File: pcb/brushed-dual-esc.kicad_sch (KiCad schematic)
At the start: 2 parts, among them J3 Conn_ARM_JTAG_SWD_10, U3 STM32C011F4Ux

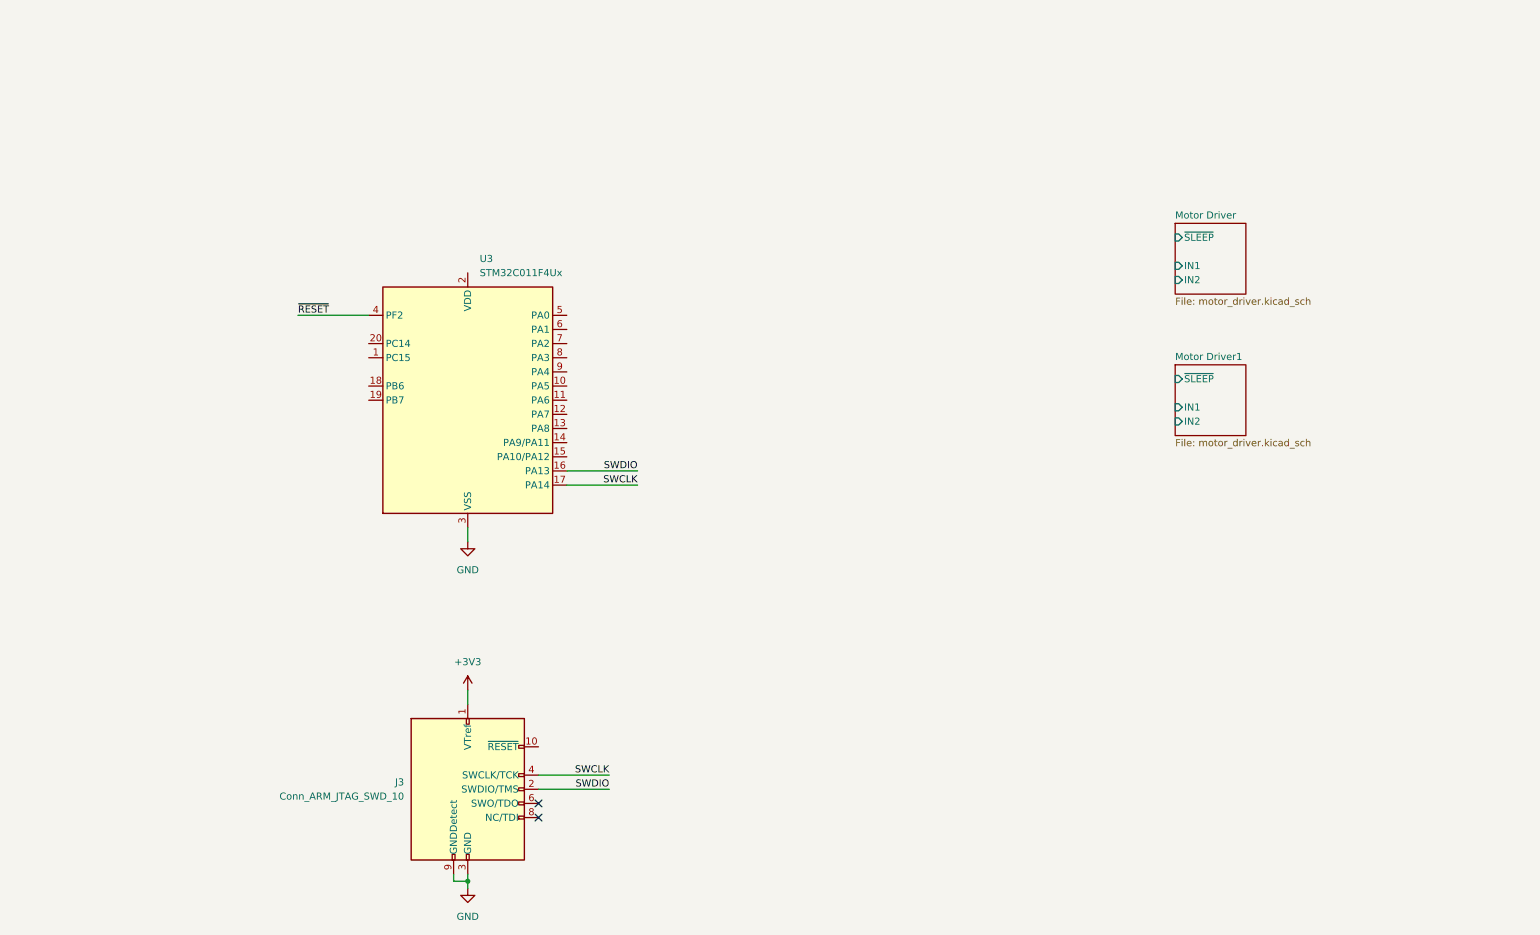
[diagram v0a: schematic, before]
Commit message: Finish design
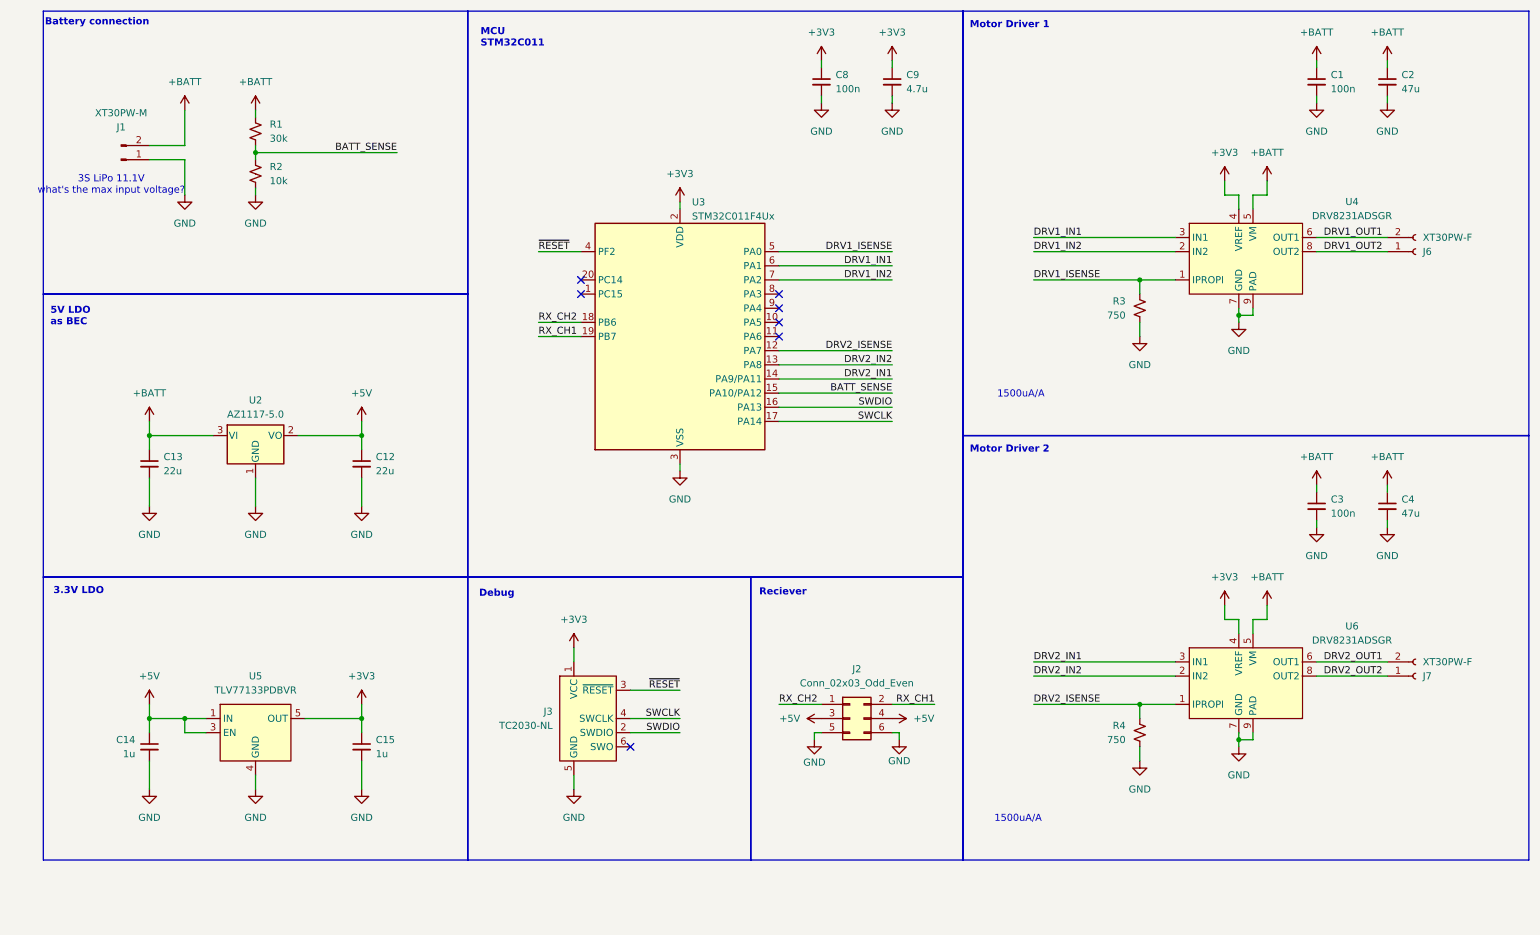
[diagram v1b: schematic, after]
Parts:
- removed J3: Conn_ARM_JTAG_SWD_10, Connector_PinHeader_1.27mm:PinHeader_2x05_P1.27mm_Vertical, symbol Connector:Conn_ARM_JTAG_SWD_10
- added C1, C3, C8: 100n, Capacitor_SMD:C_0603_1608Metric, symbol Device:C_Small
- added C12, C13: 22u, Capacitor_SMD:C_0603_1608Metric, symbol Device:C_Small
- added C14, C15: 1u, Capacitor_SMD:C_0603_1608Metric, symbol Device:C_Small
- added C2, C4: 47u, Capacitor_SMD:C_1210_3225Metric, symbol Device:C_Small
- added C9: 4.7u, Capacitor_SMD:C_0603_1608Metric, symbol Device:C_Small
- added J1: XT30PW-M, Connector_AMASS:AMASS_XT30PW-M_1x02_P2.50mm_Horizontal, symbol Connector:Conn_01x02_Pin
- added J2: Conn_02x03_Odd_Even, Connector_PinHeader_2.54mm:PinHeader_2x03_P2.54mm_Horizontal, symbol Connector_Generic:Conn_02x03_Odd_Even
- added J3: TC2030-NL, Connector:Tag-Connect_TC2030-IDC-NL_2x03_P1.27mm_Vertical, symbol Connector:Conn_ARM_SWD_TagConnect_TC2030-NL
- added J6, J7: XT30PW-F, Connector_AMASS:AMASS_XT30PW-F_1x02_P2.50mm_Horizontal, symbol Connector:Conn_01x02_Socket
- added R1: 30k, Resistor_SMD:R_0603_1608Metric, symbol Device:R_Small_US
- added R2: 10k, Resistor_SMD:R_0603_1608Metric, symbol Device:R_Small_US
- added R3, R4: 750, Resistor_SMD:R_0603_1608Metric, symbol Device:R_Small_US
- added U2: AZ1117-5.0, Package_TO_SOT_SMD:SOT-223-3_TabPin2, symbol Regulator_Linear:AZ1117-5.0
- added U4, U6: DRV8231ADSGR, Package_SON:WSON-8-1EP_2x2mm_P0.5mm_EP0.9x1.6mm, symbol Driver_Motor_TI:DRV8231ADSGR
- added U5: TLV77133PDBVR, Package_TO_SOT_SMD:SOT-23-5, symbol Regulator_Linear_TI:TLV77133PDBVR
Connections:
- net +3V3: now also U3.2 (VDD), C15.1, C8.1, C9.1, J3.1 (VCC), U4.4 (VREF), U5.5 (OUT), U6.4 (VREF)
- net GND: now also C1.2, C12.2, C13.2, C14.2, C15.2, C2.2, C3.2, C4.2, C8.2, C9.2, J1.1 (Pin_1), J2.5 (Pin_5), J2.6 (Pin_6), J3.5 (GND), R2.2, R3.2, R4.2, U2.1 (GND), U4.7 (GND), U4.9 (PAD), U5.4 (GND), U6.7 (GND), U6.9 (PAD)
- net SWCLK: now also J3.4 (SWCLK)
- net SWDIO: now also J3.2 (SWDIO)
- net ~{RESET}: now also J3.3 (~{RESET})
- net DRV2_ISENSE: now reaches U3.12 (PA7)
- net DRV2_ISENSE: now also R4.1, U6.1 (IPROPI)
- net DRV2_IN2: now reaches U3.13 (PA8)
- net DRV2_IN2: now also U6.2 (IN2)
- net DRV2_IN1: now reaches U3.14 (PA9/PA11)
- net DRV2_IN1: now also U6.3 (IN1)
- net BATT_SENSE: now reaches U3.15 (PA10/PA12)
- net BATT_SENSE: now also R1.2, R2.1
- net RX_CH2: now reaches U3.18 (PB6)
- net RX_CH2: now also J2.1 (Pin_1)
- net RX_CH1: now reaches U3.19 (PB7)
- net RX_CH1: now also J2.2 (Pin_2)
- net DRV1_ISENSE: now reaches U3.5 (PA0)
- net DRV1_ISENSE: now also R3.1, U4.1 (IPROPI)
- net DRV1_IN1: now reaches U3.6 (PA1)
- net DRV1_IN1: now also U4.3 (IN1)
- net DRV1_IN2: now reaches U3.7 (PA2)
- net DRV1_IN2: now also U4.2 (IN2)
- new net +5V: C12.1, C14.1, J2.3 (Pin_3), J2.4 (Pin_4), U2.2 (VO), U5.1 (IN), U5.3 (EN)
- new net +BATT: C1.1, C13.1, C2.1, C3.1, C4.1, J1.2 (Pin_2), R1.1, U2.3 (VI), U4.5 (VM), U6.5 (VM)
- new net DRV1_OUT1: J6.2 (Pin_2), U4.6 (OUT1)
- new net DRV1_OUT2: J6.1 (Pin_1), U4.8 (OUT2)
- new net DRV2_OUT1: J7.2 (Pin_2), U6.6 (OUT1)
- new net DRV2_OUT2: J7.1 (Pin_1), U6.8 (OUT2)
- no-connect marks 2 -> 7
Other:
- removed sheet Motor Driver
- removed sheet Motor Driver1
- note added: "1500uA/A"
- note added: "3.3V LDO"
- note added: "3S LiPo 11.1V what's the max input voltage?"
- note added: "5V LDO as BEC"
- note added: "Battery connection"
- note added: "Debug"
- note added: "MCU STM32C011"
- note added: "Motor Driver 1"
- note added: "Motor Driver 2"
- note added: "Reciever"
